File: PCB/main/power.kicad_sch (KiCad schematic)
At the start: 20 parts

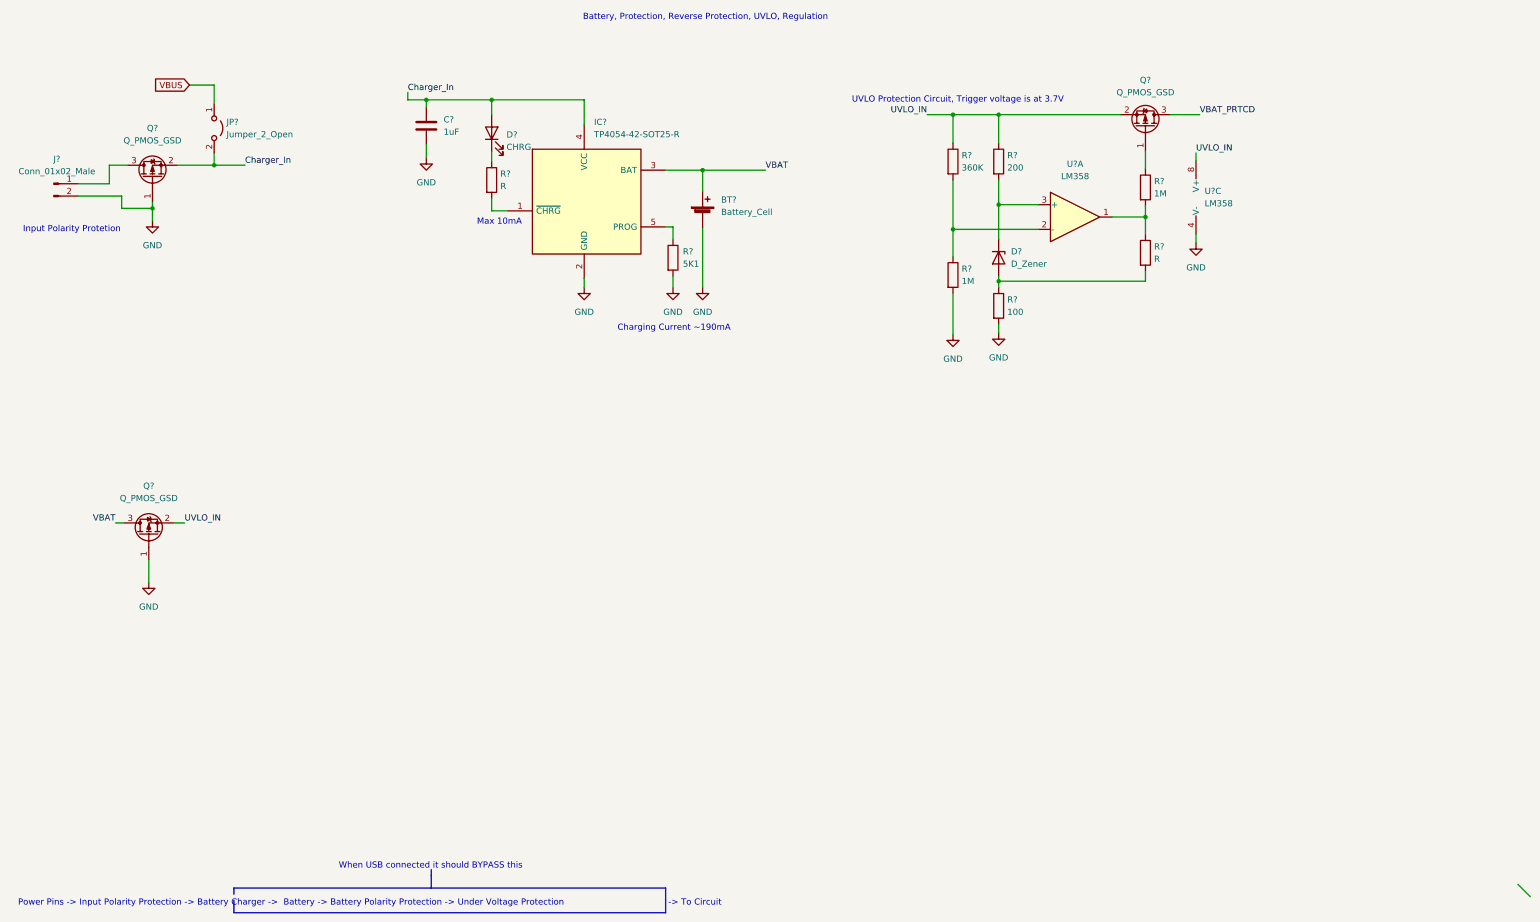
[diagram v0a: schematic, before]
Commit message: added ESD protection and updated USB IC
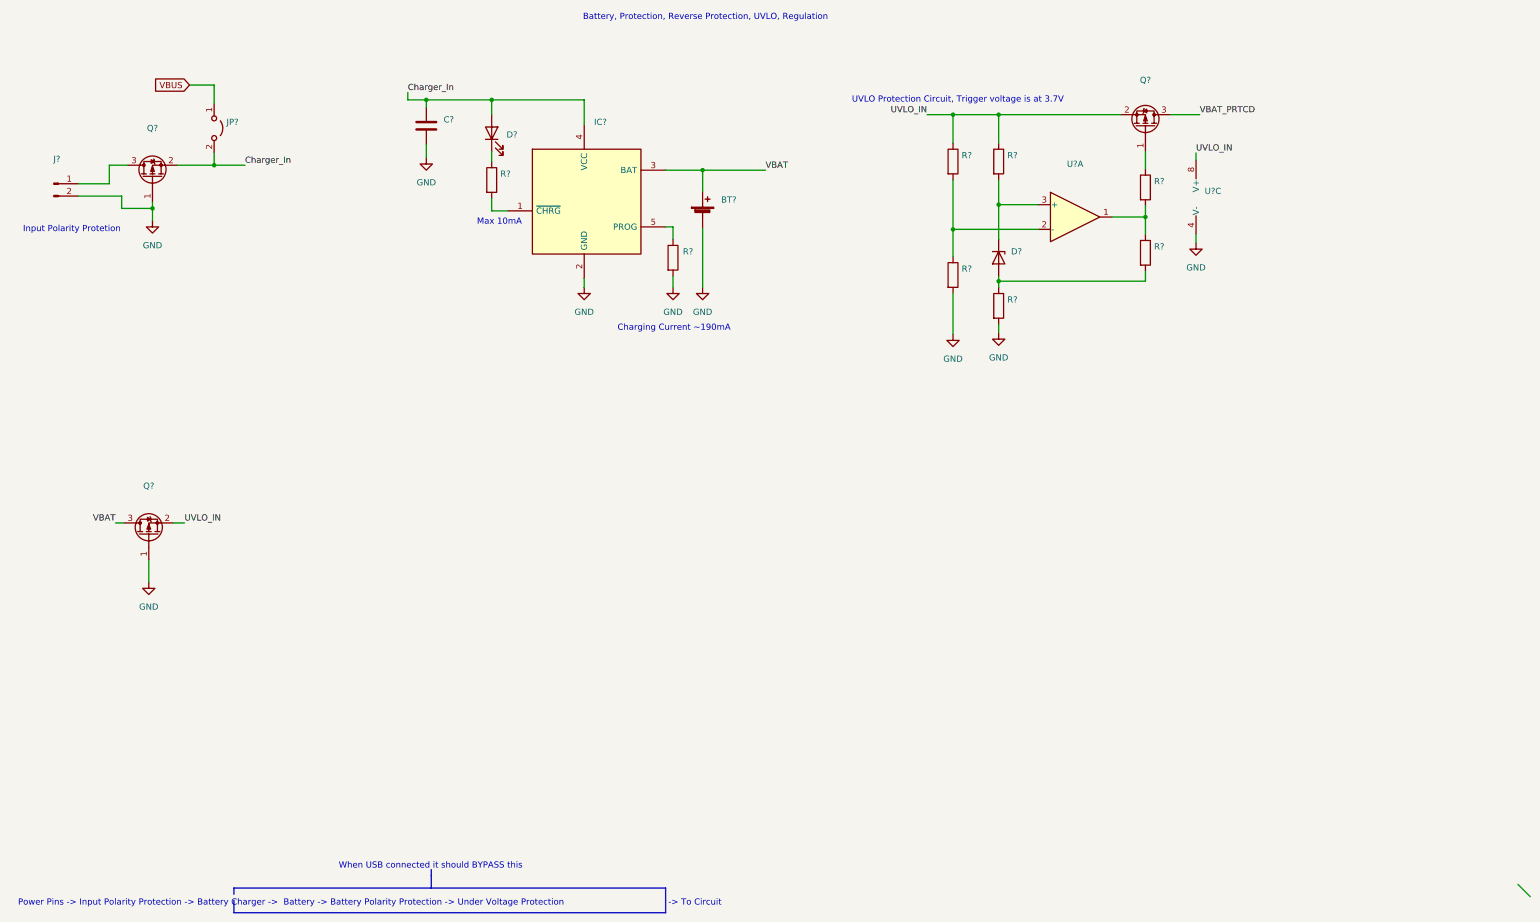
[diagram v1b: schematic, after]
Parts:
- BT?: value Battery_Cell -> (none); footprint Battery:BatteryHolder_Keystone_1042_1x18650 -> (none)
- C?: value 1uF -> (none)
- D?: value D_Zener -> (none); footprint Diode_SMD:D_SOD-523 -> (none)
- D?: value CHRG -> (none)
- IC?: value TP4054-42-SOT25-R -> (none); footprint SOT95P280X100-5N -> (none)
- J?: value Conn_01x02_Male -> (none)
- JP?: value Jumper_2_Open -> (none)
- Q? (x3): value Q_PMOS_GSD -> (none)
- R? (x2): value 1M -> (none); footprint Resistor_SMD:R_0603_1608Metric_Pad0.98x0.95mm_HandSolder -> (none)
- R?: value 5K1 -> (none); footprint Resistor_SMD:R_0805_2012Metric_Pad1.20x1.40mm_HandSolder -> (none)
- R?: value 360K -> (none); footprint Resistor_SMD:R_0603_1608Metric_Pad0.98x0.95mm_HandSolder -> (none)
- R?: value 200 -> (none); footprint Resistor_SMD:R_0603_1608Metric_Pad0.98x0.95mm_HandSolder -> (none)
- R? (x2): value R -> (none)
- R?: value 100 -> (none); footprint Resistor_SMD:R_0603_1608Metric_Pad0.98x0.95mm_HandSolder -> (none)
- U?: value LM358 -> (none)
- U?: value LM358 -> (none); footprint Package_SO:SOIC-8_3.9x4.9mm_P1.27mm -> (none)
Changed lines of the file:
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@@
     (in_bom yes) (on_board yes) (fields_autoplaced)
     (property "Reference" "Q?" (id 0) (at 252.476 20.32 90))
-    (property "Value" "Q_PMOS_GSD" (id 1) (at 252.476 22.86 90))
+    (property "Value" "" (id 1) (at 252.476 22.86 90))
     (property "Footprint" "" (id 2) (at 255.016 24.892 0)
       (effects (font (size 1.27 1.27)) hide)
@@
       (effects (font (size 1.27 1.27)) (justify left))
     )
-    (property "Value" "1M" (id 1) (at 214.63 61.7219 0)
-      (effects (font (size 1.27 1.27)) (justify left))
-    )
-    (property "Footprint" "Resistor_SMD:R_0603_1608Metric_Pad0.98x0.95mm_HandSolder" (id 2) (at 211.074 60.452 90)
+    (property "Value" "" (id 1) (at 214.63 61.7219 0)
+      (effects (font (size 1.27 1.27)) (justify left))
+    )
+    (property "Footprint" "" (id 2) (at 211.074 60.452 90)
       (effects (font (size 1.27 1.27)) hide)
     )
@@
       (effects (font (size 1.27 1.27)) (justify left))
     )
-    (property "Value" "D_Zener" (id 1) (at 224.79 58.1659 90)
-      (effects (font (size 1.27 1.27)) (justify left))
-    )
-    (property "Footprint" "Diode_SMD:D_SOD-523" (id 2) (at 222.25 56.896 0)
+    (property "Value" "" (id 1) (at 224.79 58.1659 90)
+      (effects (font (size 1.27 1.27)) (justify left))
+    )
+    (property "Footprint" "" (id 2) (at 222.25 56.896 0)
       (effects (font (size 1.27 1.27)) hide)
     )
@@
       (effects (font (size 1.27 1.27)) (justify left))
     )
-    (property "Value" "5K1" (id 1) (at 157.226 58.1659 0)
-      (effects (font (size 1.27 1.27)) (justify left))
-    )
-    (property "Footprint" "Resistor_SMD:R_0805_2012Metric_Pad1.20x1.40mm_HandSolder" (id 2) (at 153.416 56.896 90)
+    (property "Value" "" (id 1) (at 157.226 58.1659 0)
+      (effects (font (size 1.27 1.27)) (justify left))
+    )
+    (property "Footprint" "" (id 2) (at 153.416 56.896 90)
       (effects (font (size 1.27 1.27)) hide)
     )
@@
       (effects (font (size 1.27 1.27)) (justify left))
     )
-    (property "Value" "360K" (id 1) (at 214.63 38.3539 0)
-      (effects (font (size 1.27 1.27)) (justify left))
-    )
-    (property "Footprint" "Resistor_SMD:R_0603_1608Metric_Pad0.98x0.95mm_HandSolder" (id 2) (at 211.074 37.084 90)
+    (property "Value" "" (id 1) (at 214.63 38.3539 0)
+      (effects (font (size 1.27 1.27)) (justify left))
+    )
+    (property "Footprint" "" (id 2) (at 211.074 37.084 90)
       (effects (font (size 1.27 1.27)) hide)
     )
@@
       (effects (font (size 1.27 1.27)) (justify left))
     )
-    (property "Value" "LM358" (id 1) (at 264.668 45.7199 0)
+    (property "Value" "" (id 1) (at 264.668 45.7199 0)
       (effects (font (size 1.27 1.27)) (justify left))
     )
@@
       (effects (font (size 1.27 1.27)) (justify left))
     )
-    (property "Value" "TP4054-42-SOT25-R" (id 1) (at 138.9254 31.496 0)
-      (effects (font (size 1.27 1.27)) (justify left))
-    )
-    (property "Footprint" "SOT95P280X100-5N" (id 2) (at 163.83 42.672 0)
+    (property "Value" "" (id 1) (at 138.9254 31.496 0)
+      (effects (font (size 1.27 1.27)) (justify left))
+    )
+    (property "Footprint" "" (id 2) (at 163.83 42.672 0)
       (effects (font (size 1.27 1.27)) (justify left) hide)
     )
@@
     (in_bom yes) (on_board yes) (fields_autoplaced)
     (property "Reference" "U?" (id 0) (at 237.998 37.592 0))
-    (property "Value" "LM358" (id 1) (at 237.998 40.132 0))
-    (property "Footprint" "Package_SO:SOIC-8_3.9x4.9mm_P1.27mm" (id 2) (at 237.998 48.514 0)
+    (property "Value" "" (id 1) (at 237.998 40.132 0))
+    (property "Footprint" "" (id 2) (at 237.998 48.514 0)
       (effects (font (size 1.27 1.27)) hide)
     )
@@
     (in_bom yes) (on_board yes) (fields_autoplaced)
     (property "Reference" "J?" (id 0) (at 28.321 36.576 0))
-    (property "Value" "Conn_01x02_Male" (id 1) (at 28.321 39.116 0))
+    (property "Value" "" (id 1) (at 28.321 39.116 0))
     (property "Footprint" "" (id 2) (at 27.686 41.656 0)
       (effects (font (size 1.27 1.27)) hide)
@@
       (effects (font (size 1.27 1.27)) (justify left))
     )
-    (property "Value" "200" (id 1) (at 224.028 38.3539 0)
-      (effects (font (size 1.27 1.27)) (justify left))
-    )
-    (property "Footprint" "Resistor_SMD:R_0603_1608Metric_Pad0.98x0.95mm_HandSolder" (id 2) (at 220.472 37.084 90)
+    (property "Value" "" (id 1) (at 224.028 38.3539 0)
+      (effects (font (size 1.27 1.27)) (justify left))
+    )
+    (property "Footprint" "" (id 2) (at 220.472 37.084 90)
       (effects (font (size 1.27 1.27)) hide)
     )
@@
       (effects (font (size 1.27 1.27)) (justify left))
     )
-    (property "Value" "R" (id 1) (at 254.254 57.1499 0)
+    (property "Value" "" (id 1) (at 254.254 57.1499 0)
       (effects (font (size 1.27 1.27)) (justify left))
     )
@@
       (effects (font (size 1.27 1.27)) (justify left))
     )
-    (property "Value" "1M" (id 1) (at 254.254 43.6879 0)
-      (effects (font (size 1.27 1.27)) (justify left))
-    )
-    (property "Footprint" "Resistor_SMD:R_0603_1608Metric_Pad0.98x0.95mm_HandSolder" (id 2) (at 250.698 42.418 90)
+    (property "Value" "" (id 1) (at 254.254 43.6879 0)
+      (effects (font (size 1.27 1.27)) (justify left))
+    )
+    (property "Footprint" "" (id 2) (at 250.698 42.418 90)
       (effects (font (size 1.27 1.27)) hide)
     )
@@
       (effects (font (size 1.27 1.27)) (justify right))
     )
-    (property "Value" "CHRG" (id 1) (at 120.904 34.0994 90)
+    (property "Value" "" (id 1) (at 120.904 34.0994 90)
       (effects (font (size 1.27 1.27)) (justify right))
     )
@@
       (effects (font (size 1.27 1.27)) (justify left))
     )
-    (property "Value" "Jumper_2_Open" (id 1) (at 63.246 31.4959 90)
+    (property "Value" "" (id 1) (at 63.246 31.4959 90)
       (effects (font (size 1.27 1.27)) (justify left))
     )
@@
     (in_bom yes) (on_board yes) (fields_autoplaced)
     (property "Reference" "Q?" (id 0) (at 48.006 30.226 90))
-    (property "Value" "Q_PMOS_GSD" (id 1) (at 48.006 32.766 90))
+    (property "Value" "" (id 1) (at 48.006 32.766 90))
     (property "Footprint" "" (id 2) (at 45.466 35.306 0)
       (effects (font (size 1.27 1.27)) hide)
@@
       (effects (font (size 1.27 1.27)) (justify left))
     )
-    (property "Value" "R" (id 1) (at 119.634 42.1639 0)
+    (property "Value" "" (id 1) (at 119.634 42.1639 0)
       (effects (font (size 1.27 1.27)) (justify left))
     )
@@
       (effects (font (size 1.27 1.27)) (justify left))
     )
-    (property "Value" "Battery_Cell" (id 1) (at 165.1 47.4979 0)
-      (effects (font (size 1.27 1.27)) (justify left))
-    )
-    (property "Footprint" "Battery:BatteryHolder_Keystone_1042_1x18650" (id 2) (at 161.29 46.736 90)
+    (property "Value" "" (id 1) (at 165.1 47.4979 0)
+      (effects (font (size 1.27 1.27)) (justify left))
+    )
+    (property "Footprint" "" (id 2) (at 161.29 46.736 90)
       (effects (font (size 1.27 1.27)) hide)
     )
@@
     (in_bom yes) (on_board yes) (fields_autoplaced)
     (property "Reference" "Q?" (id 0) (at 47.244 103.886 90))
-    (property "Value" "Q_PMOS_GSD" (id 1) (at 47.244 106.426 90))
+    (property "Value" "" (id 1) (at 47.244 106.426 90))
     (property "Footprint" "" (id 2) (at 44.704 108.966 0)
       (effects (font (size 1.27 1.27)) hide)
@@
       (effects (font (size 1.27 1.27)) (justify left))
     )
-    (property "Value" "1uF" (id 1) (at 107.95 30.9879 0)
+    (property "Value" "" (id 1) (at 107.95 30.9879 0)
       (effects (font (size 1.27 1.27)) (justify left))
     )
@@
       (effects (font (size 1.27 1.27)) (justify left))
     )
-    (property "Value" "100" (id 1) (at 224.028 68.0719 0)
-      (effects (font (size 1.27 1.27)) (justify left))
-    )
-    (property "Footprint" "Resistor_SMD:R_0603_1608Metric_Pad0.98x0.95mm_HandSolder" (id 2) (at 220.472 66.802 90)
-      (effects (font (size 1.27 1.27)) hide)
-    )
+    (property "Value" "" (id 1) (at 224.028 68.0719 0)
+      (effects (font (size 1.27 1.27)) (justify left))
+    )
+    (property "Footprint" "" (id 2) (at 220.472 66.802 90)
+      (effects (font (size 1.27 1.27)) hide)
+    )
